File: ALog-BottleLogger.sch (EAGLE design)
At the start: 88 parts, among them IC1 24AA256SN, J6 5.5x2.1mm Barrel, Q5 4.3A/20V/54mΩ, Q6 4.3A/20V/54mΩ, Q7 4.3A/20V/54mΩ, Q8 220mA/50V/3.5Ω, Q9 220mA/50V/3.5Ω, U1 ATSAMD21G-A, U4 SX1509

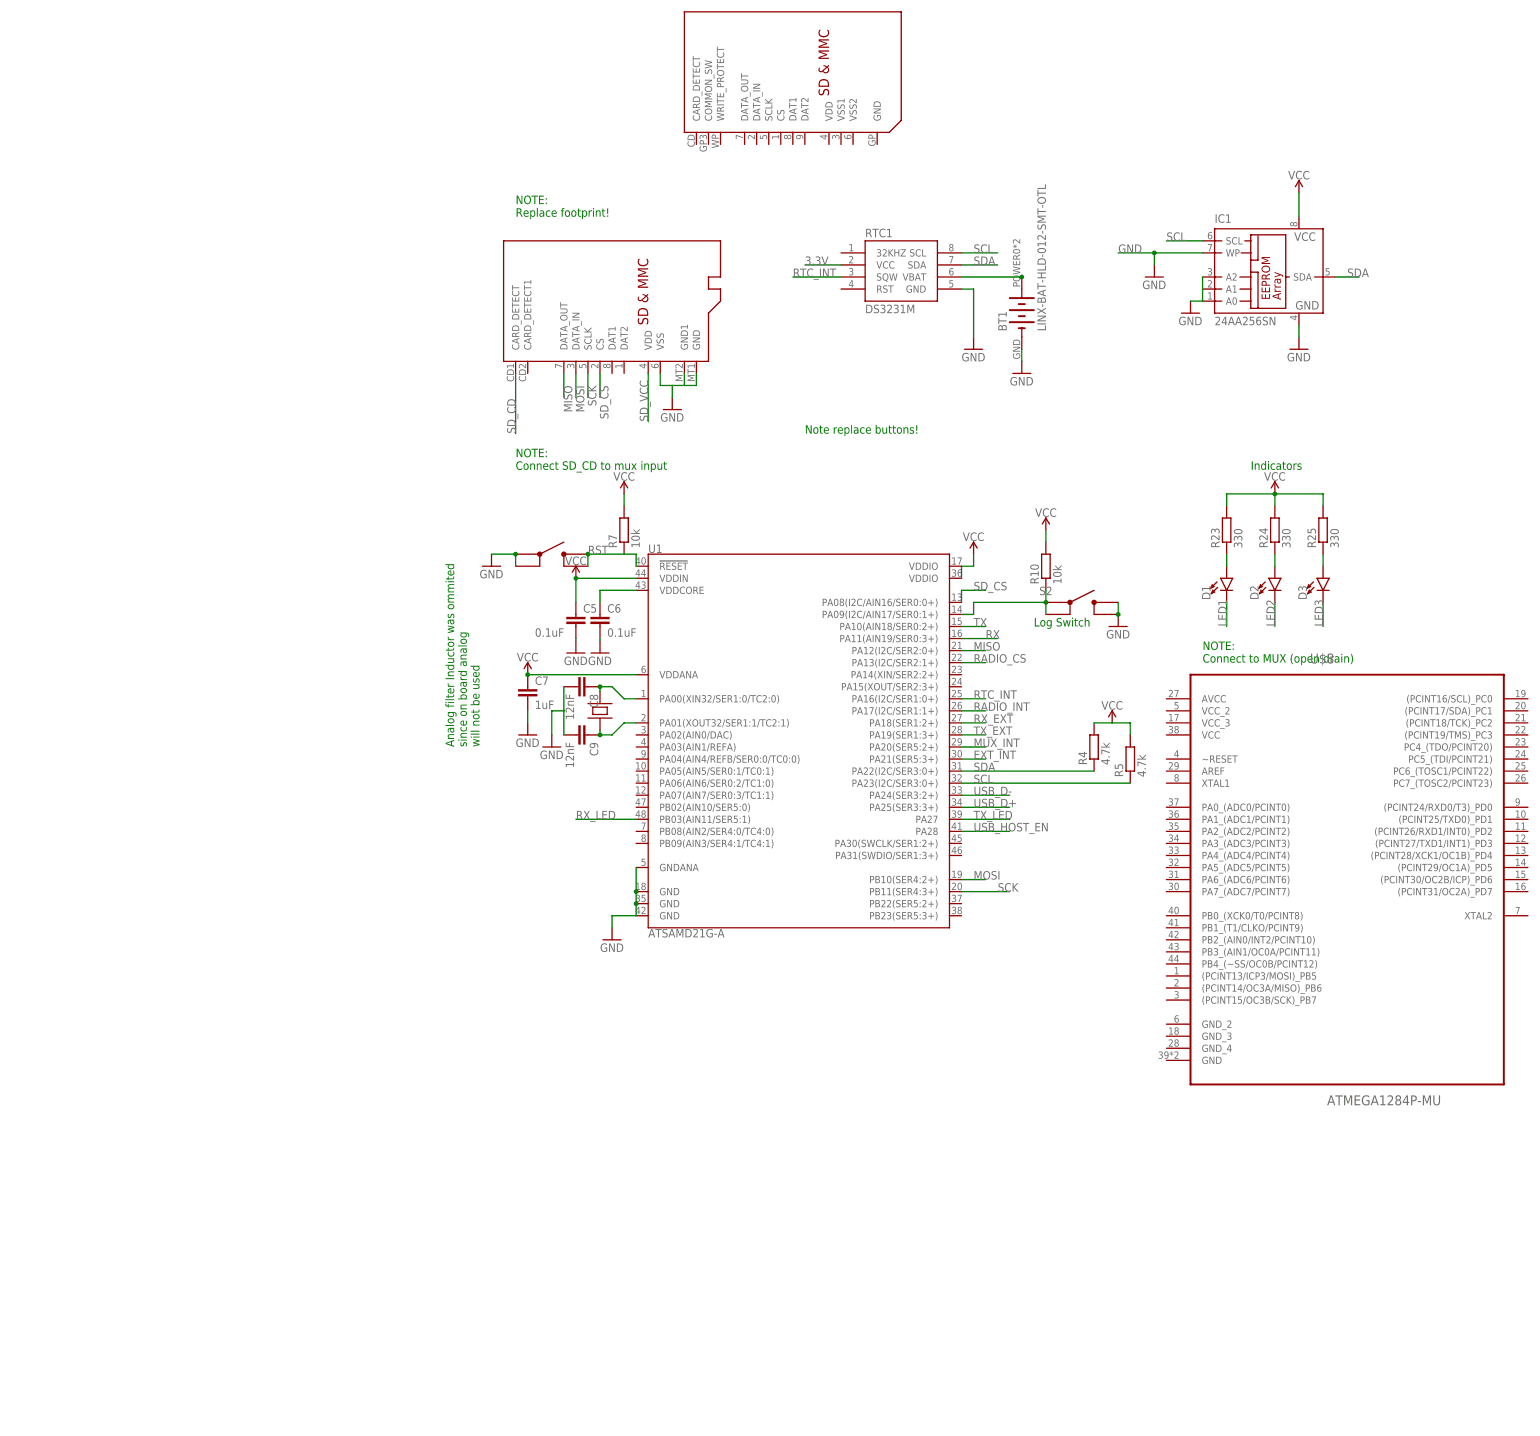
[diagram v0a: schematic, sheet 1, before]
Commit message: Work in progress
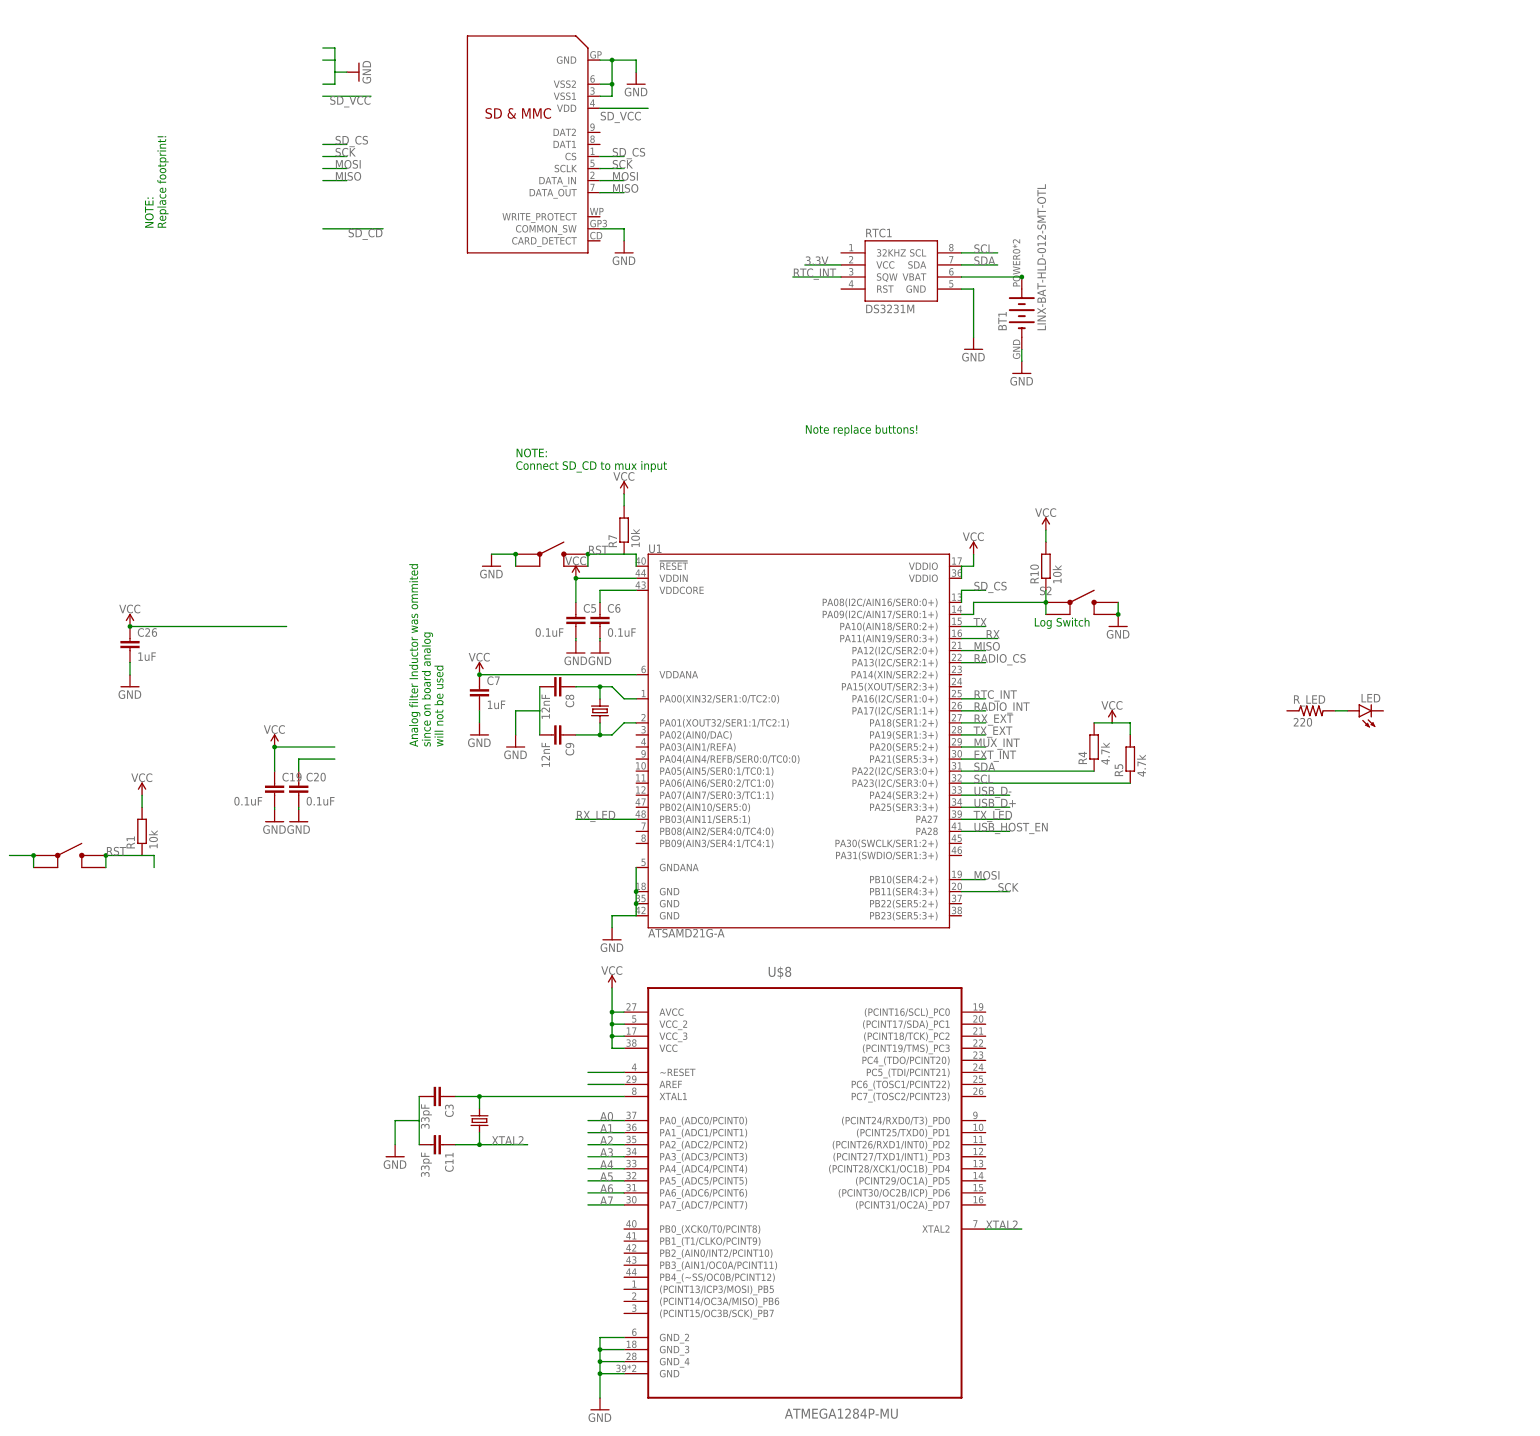
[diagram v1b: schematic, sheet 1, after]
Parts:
- removed D1, D2, D3: (no value), SparkFun-LED:LED0603
- removed F1, F2: 6V/0.5A, SparkFun-Fuses:PPTC_HALF-AMP
- removed IC1: 24AA256SN, microchip:24AA256SN
- removed R11, R12: 10k, rcl:R-EU_R0603
- removed R2: 383k, rcl:R-EU_R0603
- removed R23, R24, R25, R39: 330, rcl:R-EU_R0603
- removed R38: 100k, rcl:R-EU_R0603
- removed U$2: MICROSD, adafruit:MICROSD
- removed U$5: CM200, Custom:CM200
- removed U4: SX1509, SparkFun-IC-Special-Function:SX1509
- added C19, C20: 0.1uF, rcl:C-EUC0603
- added C26: 1uF, rcl:C-EUC0603
- added C3: 33pF, rcl:C-EUC0603
- added F3, F4: 6V/0.5A, SparkFun-Fuses:PPTC_HALF-AMP
- added J12, J13: (no value), SparkFun-Connectors:M08SMD-STRAIGHT-FEMALE
- added J14, J15, J16: (no value), SparkFun-Connectors:CONN_10
- added J17: (no value), SparkFun-Connectors:M11SMD_NO_HOLES
- added LED: (no value), SparkFun-LED:LED1206
- added Q1, Q2: (no value), crystal:CRYSTALHC49UP
- added R_LED: 220, resistor:R-US_R0603
- added U$4: SKRPABE010, Custom:SKRPABE010
- C11: value 0.1uF -> 33pF
- C4: value 2.2uF -> 10nF; device rcl:C-EUC0603 -> rc-master-smd:CCA_
- J10: device SparkFun-Connectors:CONN_10 -> SparkFun-Connectors:M102MMSMD
- J5, J9: device SparkFun-Connectors:CONN_10 -> SparkFun-Connectors:M08SMD-STRAIGHT-FEMALE
- R1: value 2M -> 10k
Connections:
- removed net EXT_D6: J10.7, U4.I/O[10]
- removed net GPIO_EXT1: J5.1, U4.I/O[12]
- removed net GPIO_EXT2: J5.2, U4.I/O[13]
- removed net GPIO_EXT3: J5.3, U4.I/O[14]
- removed net GPIO_EXT4: J5.4, U4.I/O[15]
- removed net LED1: D1.C, U4.I/O[5]
- removed net LED2: D2.C, U4.I/O[6]
- removed net LED3: D3.C, U4.I/O[7]
- removed net N$14: F1.1, Q5.D
- removed net N$18: F2.1, Q6.D
- removed net N$27: U4.OSCIO
- removed net N$32: D1.A, R23.1
- removed net N$33: D2.A, R24.1
- removed net N$34: D3.A, R25.1
- removed net N$50: J3.ID, R38.1, R39.2
- removed net N$53: R44.1, R45.2, U$7.CH15
- removed net N$54: R46.1, R47.1, U$7.CH14
- removed net N$56: R11.1, U4.!RESET
- removed net SD_CD: U$2.CARD_DETECT
- removed net SPI_EXT_CS1: U4.I/O[11]
- removed net SPI_EXT_CS2: J10.6, U4.I/O[9]
- new net A0: U$8.PA0_(ADC0/PCINT0)
- new net A1: U$8.PA1_(ADC1/PCINT1)
- new net A2: U$8.PA2_(ADC2/PCINT2)
- new net A3: U$8.PA3_(ADC3/PCINT3)
- new net A4: U$8.PA4_(ADC4/PCINT4)
- new net A5: U$8.PA5_(ADC5/PCINT5)
- new net A6: U$8.PA6_(ADC6/PCINT6)
- new net A7: U$8.PA7_(ADC7/PCINT7)
- new net ADC12: J14.7, U$7.CH12
- new net ADC13: J14.6, U$7.CH13
- new net ADC14: J14.2, R46.1, R47.1, U$7.CH14
- new net ADC15: J14.1, R44.1, R45.2, U$7.CH15
- new net EXT_3.3V1: J14.4, J15.4, J16.7, J8.7
- new net EXT_5V1: J14.5, J15.5, J16.8, J8.8
- new net GND1: U$4.1
- new net GND2: C4A.2, C4B.2, C4C.2, C4D.2
- new net GND3: J14.3, J15.3, J16.6, J8.6
- new net LED+: LED.A, R_LED.2
- new net N$17: F3.1, Q5.D
- new net N$2: U$8.~RESET
- new net N$23: F4.1, Q6.D
- new net N$4: U$8.AREF
- new net N$6: C20.1
- new net XTAL2: C11.1, Q2.1, U$8.XTAL2
- net 3.3V: now also C19.1, C26.1, R1.2, R44.2; no longer C11.1, IC1.VCC, R1.1, R11.2, R12.2, R23.2, R24.2, R25.2, U4.VCC1, U4.VCC2, U4.VDDM
- net 3.3V_EXT_CTRL: no longer U4.I/O[8]
- net 5V: no longer C4.1, R38.2, R44.2
- net 5V_EXT_CTRL: no longer U4.I/O[4]
- net ADC0: now also J8.4; no longer J8.2
- net ADC1: now also J8.5; no longer J8.4
- net ADC10: now also J15.2; no longer J5.9
- net ADC11: now also J15.1; no longer J5.10
- net ADC2: now also J8.9; no longer J8.6
- net ADC3: now also J8.10; no longer J8.8
- net ADC4: now also J16.4; no longer J8.10
- net ADC5: now also J16.5; no longer J9.2
- net ADC6: now also J16.9; no longer J5.5
- net ADC7: now also J16.10; no longer J5.6
- net ADC8: now also J15.7; no longer J5.7
- net ADC9: now also J15.6; no longer J5.8
- net EXT_3.3V: now also F3.2, J14.9, J15.9, J16.2, J8.2; no longer F1.2, J10.5, J10.8, J8.3, J8.5, J8.9, J9.1, J9.5
- net EXT_5V: now also F4.2, J14.10, J15.10, J16.3, J8.3; no longer F2.2, J10.9, J9.4
- net EXT_INT: no longer J9.3
- net GND: now also C19.2, C20.2, C26.2, C3.2, J14.8, J15.8, J16.1, SD.COMMON_SW, SD.GND, SD.VSS1, SD.VSS2, U$3.FB, U$8.GND, U$8.GND_2, U$8.GND_3, U$8.GND_4; no longer C4.2, IC1.A0, IC1.A1, IC1.A2, IC1.GND, IC1.WP, J10.1, J10.10, J8.7, J9.6, R2.2, U$2.GND, U$2.GND1, U$2.VSS, U4.ADDR0, U4.ADDR1, U4.GND
- net MISO: no longer J10.2, U$2.DATA_OUT
- net MOSI: no longer J10.3, U$2.DATA_IN
- net MUX_INT: no longer R12.1, U4.!INT
- net N$10: now also Q1.1; no longer U$5.P$1
- net N$3: now also C3.1, Q2.2; no longer R1.2, R2.1, U$3.FB
- net N$9: now also Q1.2; no longer U$5.P$2
- net RST: now also R1.1, U$4.3
- net RX_EXT: no longer J9.7
- net SCK: no longer J10.4, U$2.SCLK
- net SCL: no longer IC1.SCL, J9.10, U4.SCL
- net SDA: no longer IC1.SDA, J9.9, U4.SDA
- net SD_CS: no longer U$2.CS
- net SD_VCC: no longer U$2.VDD
- net SD_VCC_CTRL: no longer U4.I/O[2]
- net TX_EXT: no longer J9.8
- net USB_HOST_EN: no longer R39.1
- net VCC: now also U$8.AVCC, U$8.VCC, U$8.VCC_2, U$8.VCC_3
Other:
- note added: "3.3V TPS62172"
- note added: "NOTE: Why was Bobby measuring the 5V input, should we measure 3.3V?"
- note removed: "5v TPS62175"
- note removed: "Indicators"
- note removed: "NOTE: Connect to MUX (open drain)"
- note removed: "NOTE: Get info from Ying!"
- note removed: "SUBNOTE: Fix resistor values"
- moved on the sheet: C7, C8, C9, J1, J2, J8, Q5, Q6, R20, R21, R44, R45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
